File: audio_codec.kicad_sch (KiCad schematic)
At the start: 38 parts, among them J200 Headphones, J201 AudioInput, J202 AudioOutput, U200 WM8731SEDS, U201 TPA6110A2DGN

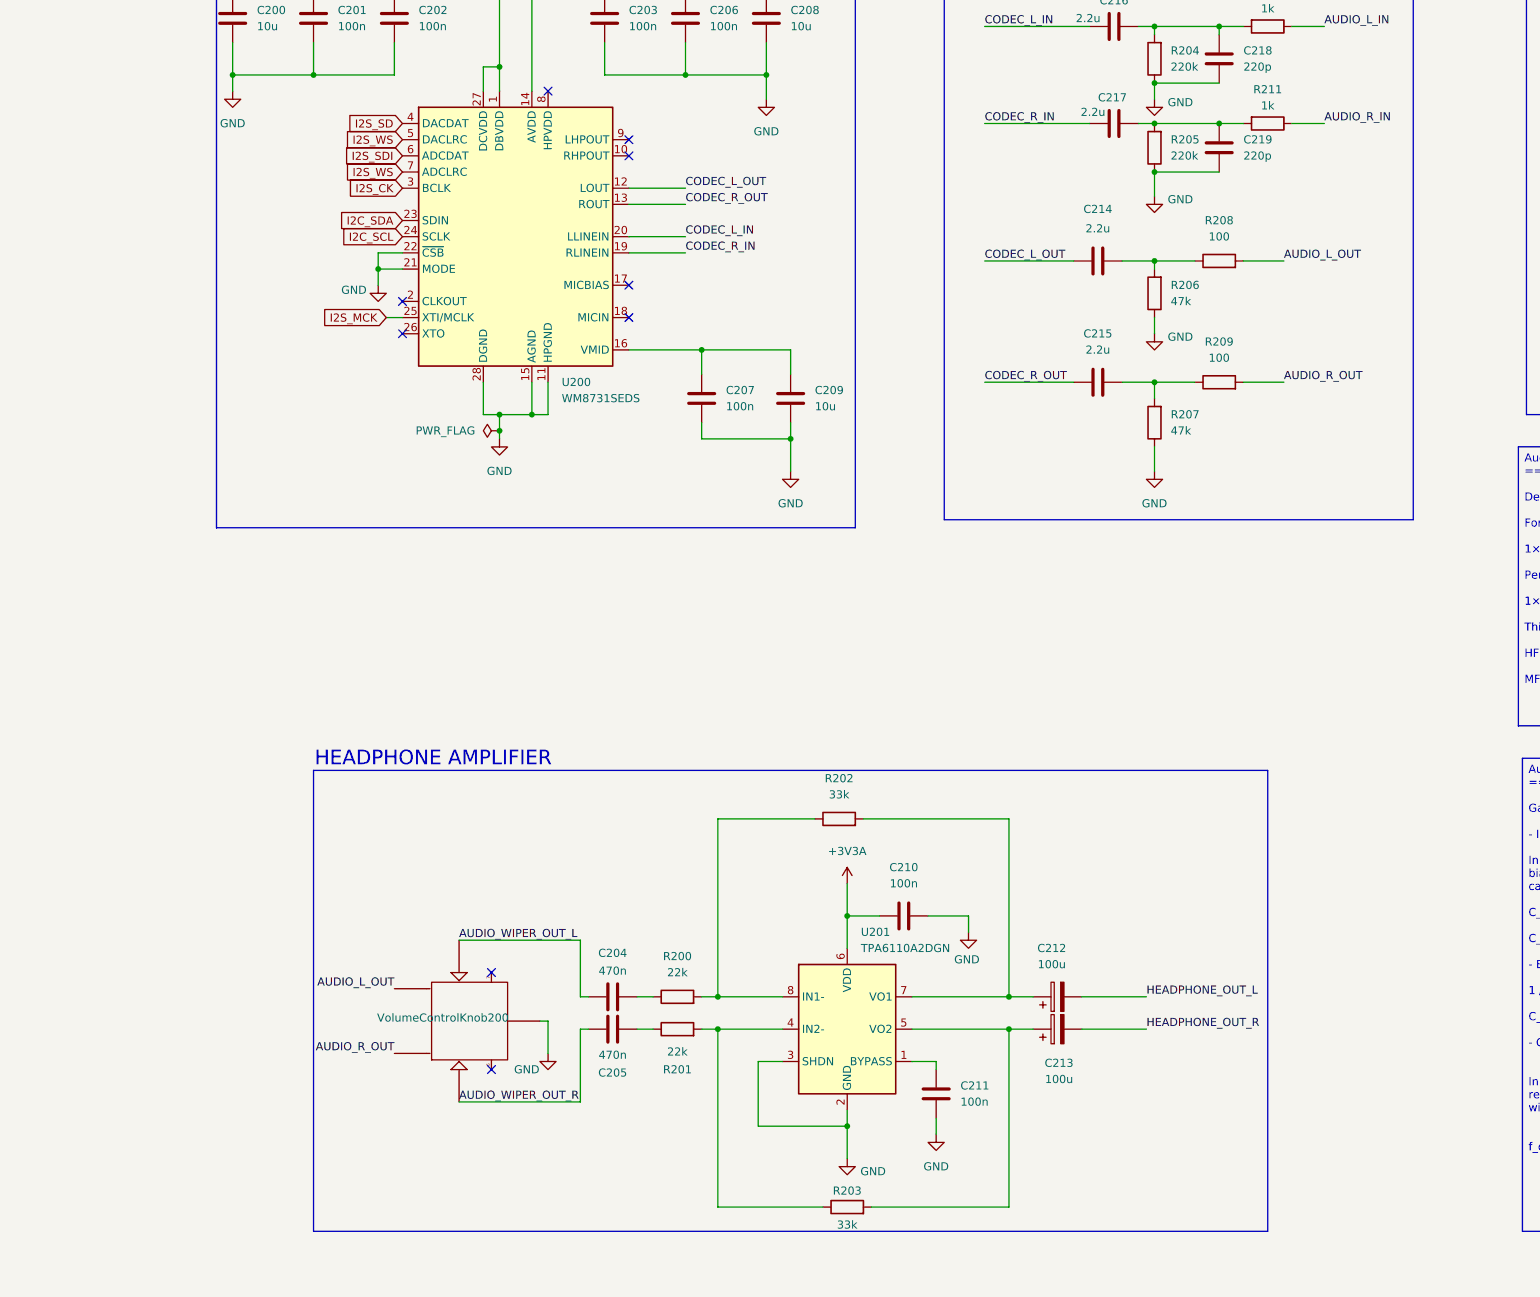
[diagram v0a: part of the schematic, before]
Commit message: updating names
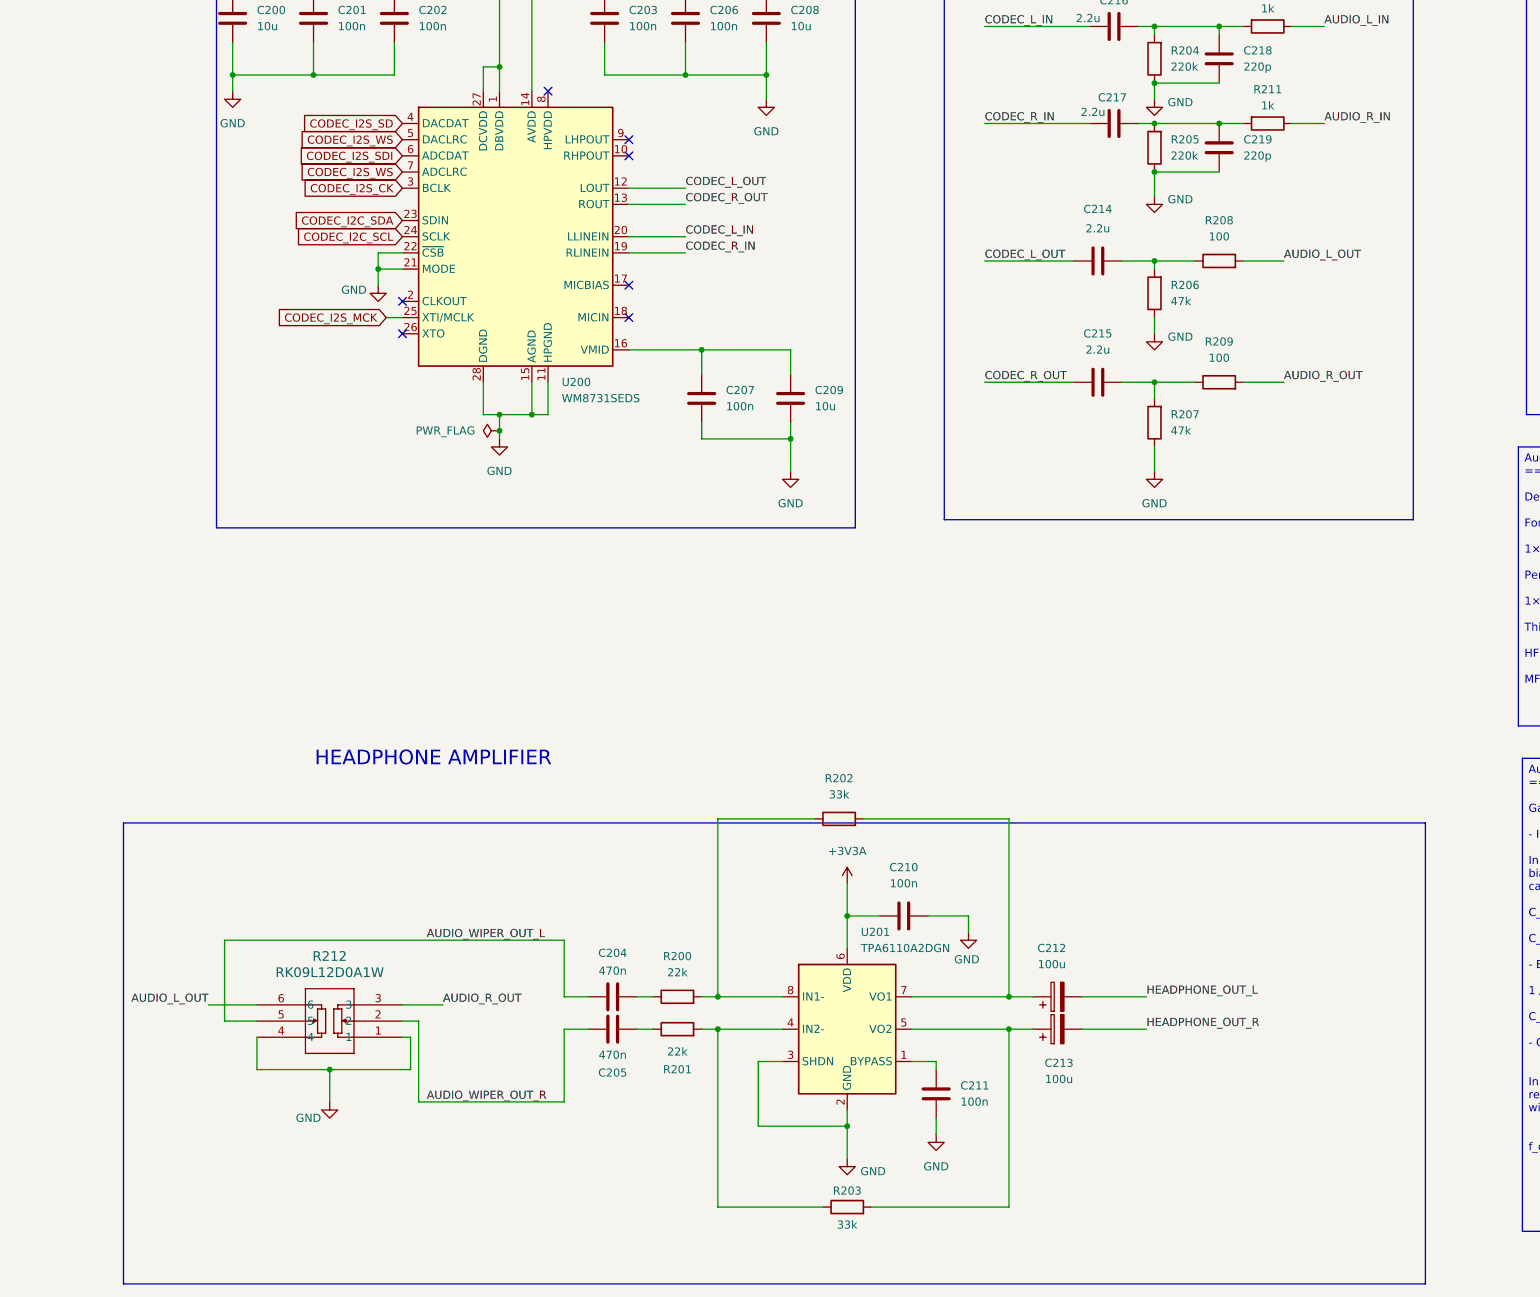
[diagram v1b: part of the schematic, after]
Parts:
- removed VolumeControlKnob200: ~, Galerna:RK10J12R0A0B, symbol Galerna:RK10J12R0A0B
- added R212: RK09L12D0A1W, Galerna:RK09L12D0A1W_AAL, symbol Galerna:RK09L12D0A1W
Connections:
- net AUDIO_L_OUT: now also R212.6
- net AUDIO_R_OUT: now also R212.3
- net AUDIO_WIPER_OUT_L: now also R212.5
- net AUDIO_WIPER_OUT_R: now also R212.2
- net GND: now also R212.1, R212.4
- net I2C_SCL renamed CODEC_I2C_SCL
- net I2C_SDA renamed CODEC_I2C_SDA
- net I2S_CK renamed CODEC_I2S_CK
- net I2S_MCK renamed CODEC_I2S_MCK
- net I2S_SD renamed CODEC_I2S_SD
- net I2S_SDI renamed CODEC_I2S_SDI
- net I2S_WS renamed CODEC_I2S_WS
- no-connect marks 12 -> 10
